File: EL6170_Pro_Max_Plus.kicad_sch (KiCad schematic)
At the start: 56 parts, among them J1 USB_C_Receptacle, Q1 MMBT3904, Q2 MMBT3904, SW1 RST, SW2 BOOT, U1 ESP32-S3, U3 ESP-PSRAM64H, U4 W25Q128JVS, U5 ME6217C33M5, U6 CH340K, U7 RFANT5220110A0T, U8 CH334R, X1 40MHz, X2 12MHz

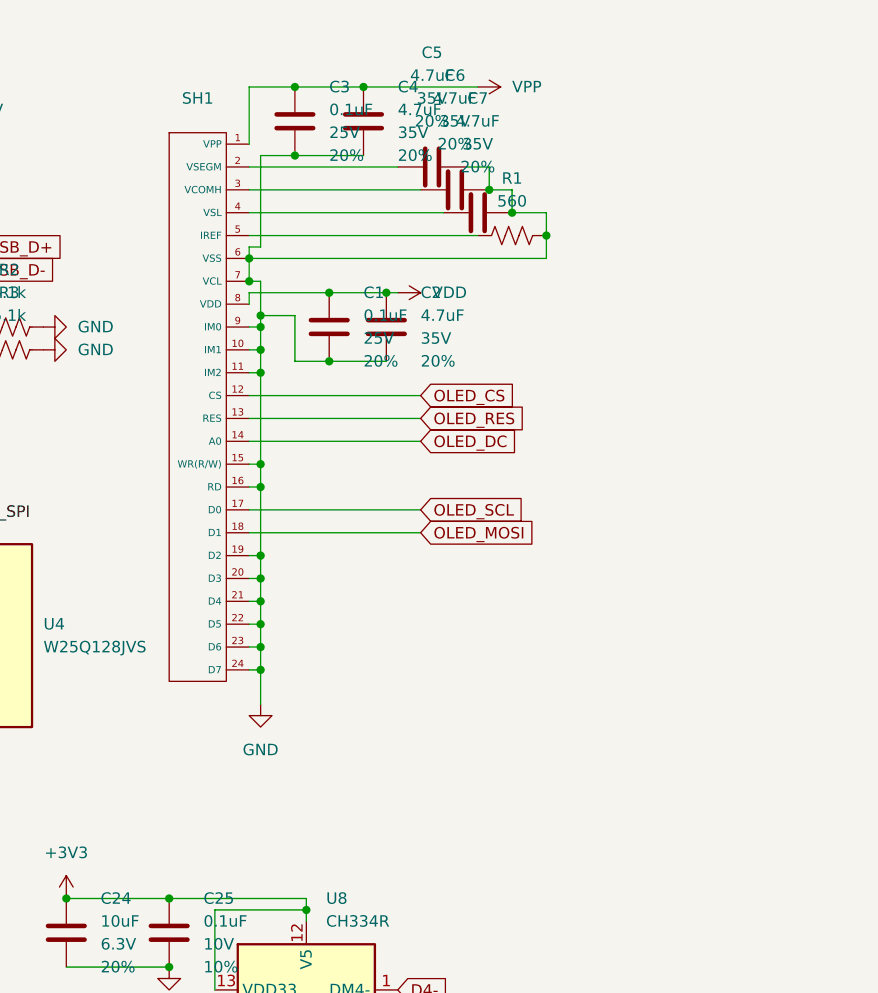
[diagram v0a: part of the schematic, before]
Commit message: sync
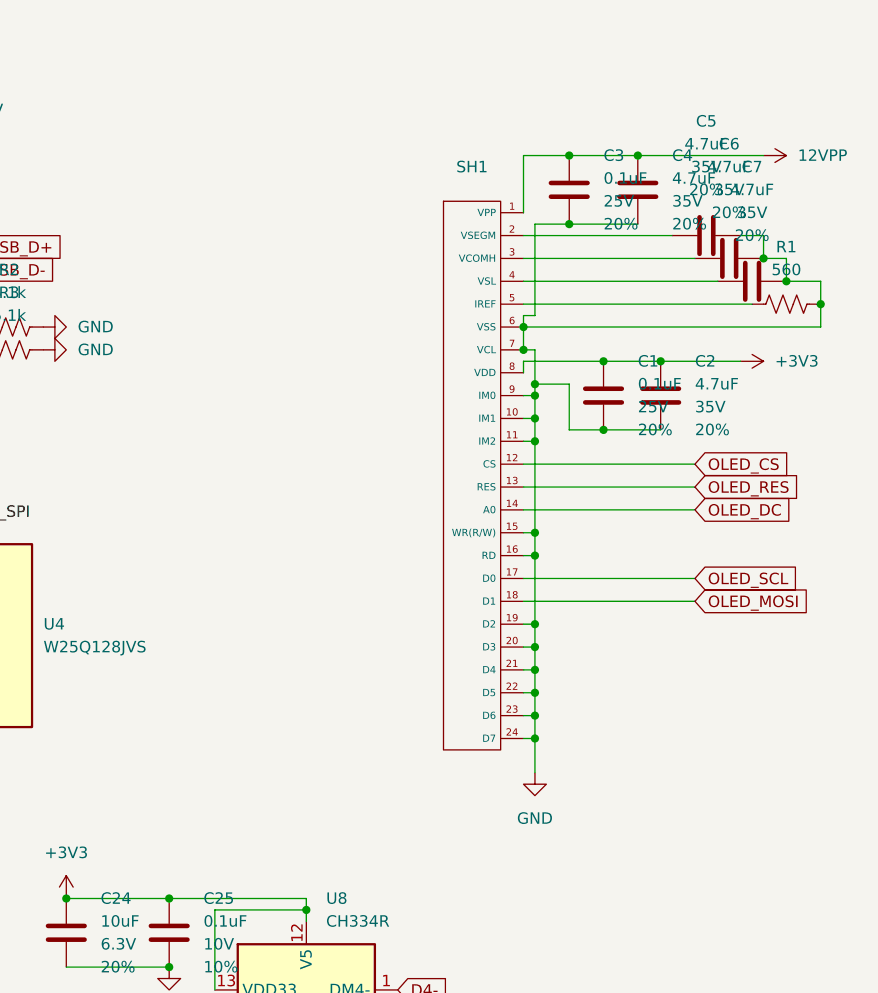
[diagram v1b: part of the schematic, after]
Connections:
- net VDD is gone; now on net +3V3: C1.1, C2.1, SH1.8 (VDD)
- net VPP renamed 12VPP
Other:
- moved on the sheet: C1, C2, C3, C4, C5, C6, C7, R1, SH1
